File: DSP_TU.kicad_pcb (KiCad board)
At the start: 4 copper layers, 165.1 x 114.3 mm, 83 parts, among them J1 Conn_01x07_Male, J2 Conn_01x08_Male, J3 USB_B, J4 Conn_01x08_Male, J5 1757569, J6 Conn_01x08_Male, J7 Conn_01x08_Male, K1 G3VM-601BY, K2 G3VM-601BY, T1 TY-141P, T2 TY-145P, U1 PIC32MZ0512EFE064-I_PT, U2 TLV2780CDBVT, U3 FT231XS-U, U4 H11AA1, U5 74HCT2G14GW-Q100H, U6 AP2112K-3.3, U7 ATWINC1510-MR210UB, U8 W25X40CLSN

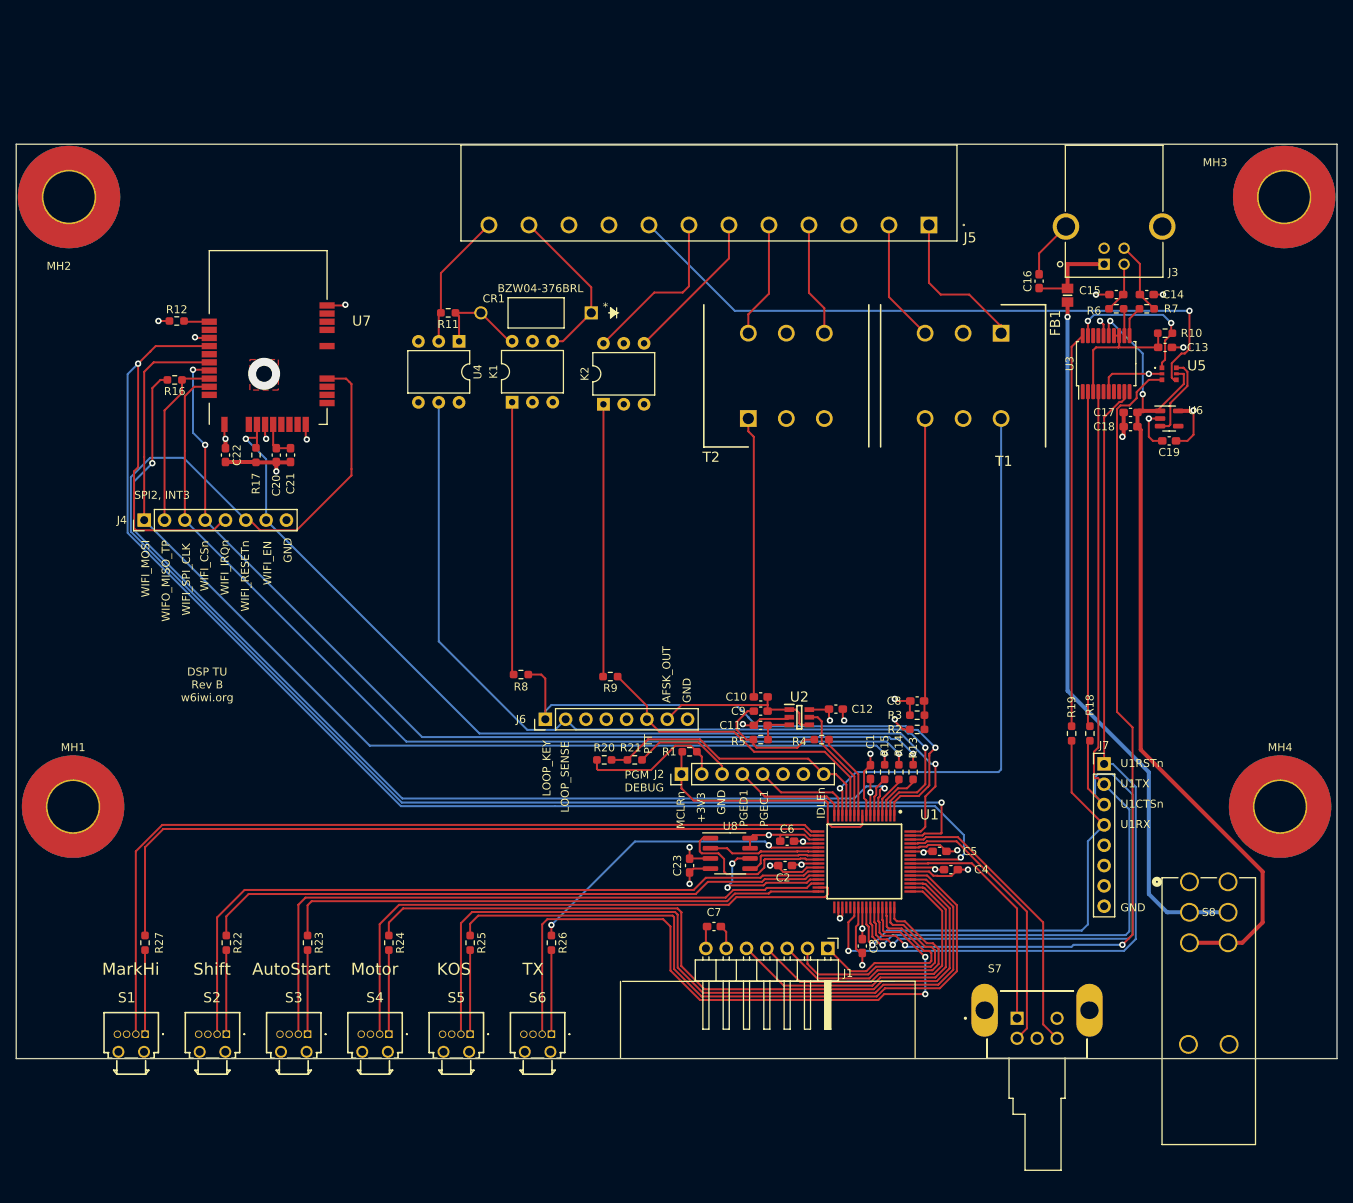
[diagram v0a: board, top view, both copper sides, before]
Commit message: Update all to rev C
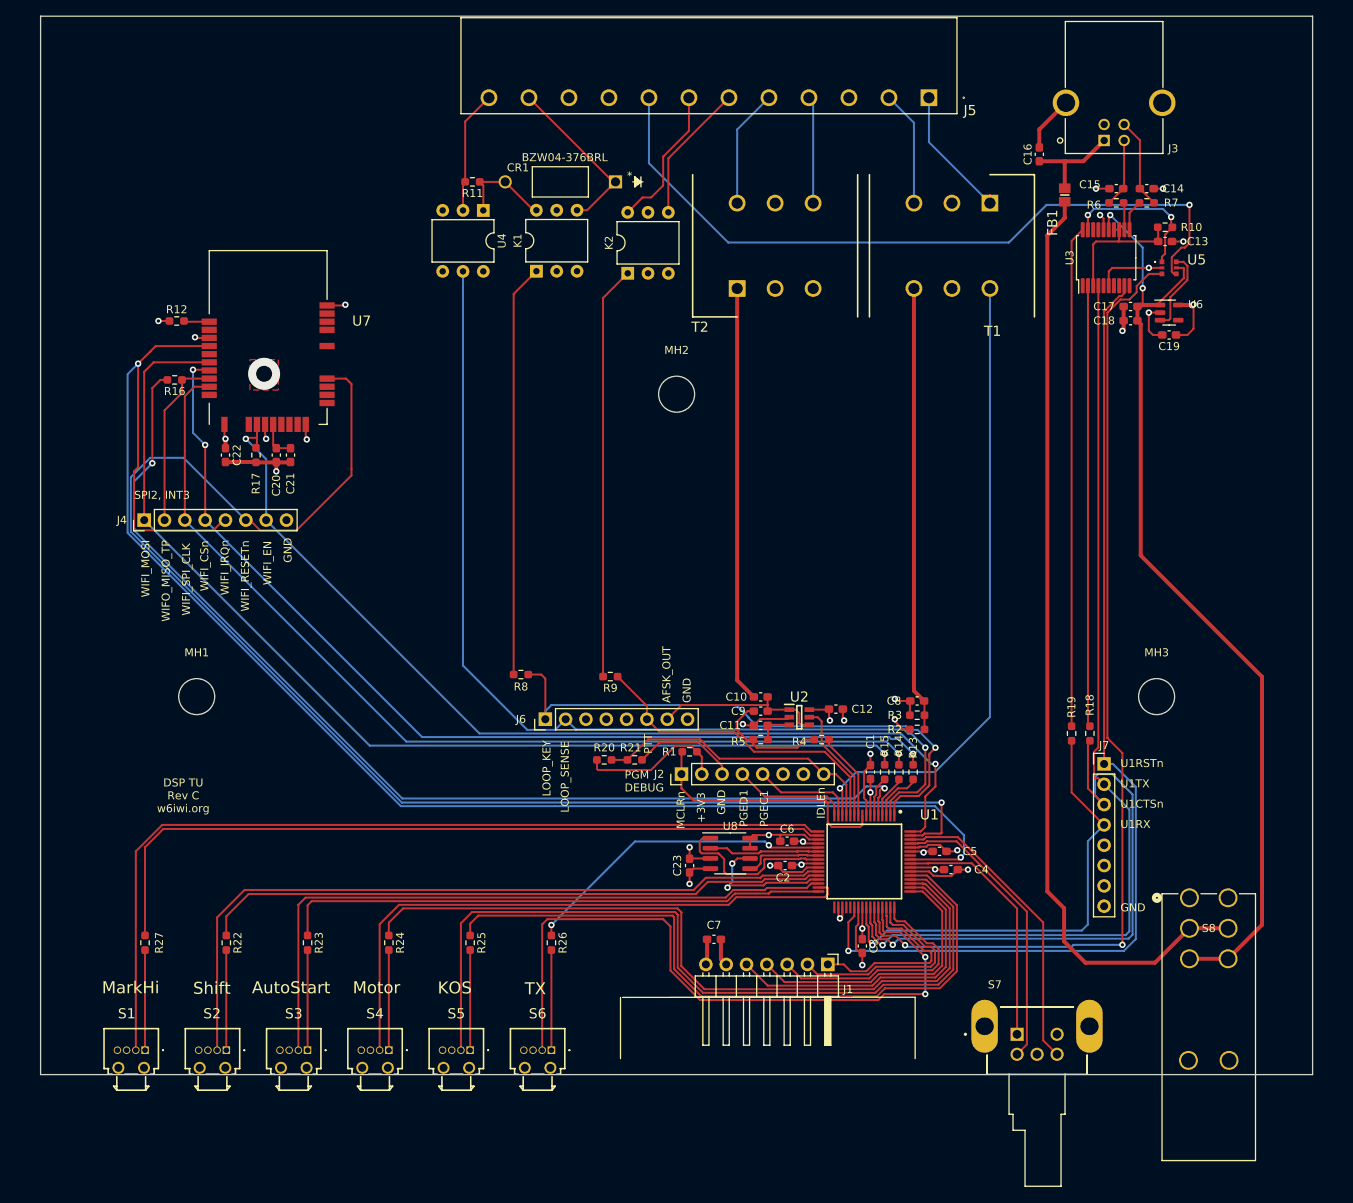
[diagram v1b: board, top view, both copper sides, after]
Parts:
- removed MH4: MountingHole_6.4mm_M6_Pad_TopBottom, MountingHole:MountingHole_6.4mm_M6_Pad_TopBottom
- MH1, MH2, MH3: value MountingHole_6.4mm_M6_Pad_TopBottom -> MountingHole_4.5mm; footprint MountingHole:MountingHole_6.4mm_M6_Pad_TopBottom -> MountingHole:MountingHole_4.5mm
- moved MH2 79.8 mm to (116.6, 60.5)
- moved MH3 64.4 mm to (176.6, 98.3)
- moved MH1 20.7 mm to (56.6, 98.3)
- moved K2 16.7 mm to (110.5, 45.3)
- moved R11 16.7 mm to (91.1, 33.9)
- moved CR1 16.7 mm to (109.0, 33.9)
- moved K1 16.7 mm to (99.1, 45.1)
- moved U4 16.7 mm to (92.4, 37.5)
- moved T1 16.3 mm to (155.8, 36.6)
- moved T2 16.3 mm to (124.2, 47.2)
- moved J5 15.9 mm to (148.1, 23.4)
- moved C16 15.8 mm to (161.9, 30.5)
- moved J3 15.5 mm to (170.0, 28.7)
- moved C18 13.2 mm to (173.3, 51.3)
- moved C13 13.2 mm to (177.6, 41.4)
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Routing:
- net +5V: track 89.1 -> 117.6 mm, vias 1 -> 0
- net Net-(K1-Pad1): track 34.1 -> 51.9 mm
- net Net-(K2-Pad1): track 34.1 -> 51.8 mm
- net Net-(T1-SEC_1): track 39.3 -> 56.2 mm
- net Net-(C10-Pad1): track 35.1 -> 51.9 mm
- net LOOP_SENSE: track 108.9 -> 124.1 mm
- net +5V_SW: track 105.2 -> 119.4 mm
- net U1RTSn: track 114.2 -> 127.4 mm
- net U1TX: track 106.9 -> 120.1 mm
- net Net-(U3-TXD): track 49.4 -> 62.6 mm
- net Net-(U3-RTS#): track 41.9 -> 55.2 mm
- net AUTOSTARTn: track 110.3 -> 123.5 mm
- net Net-(T1-SEC_3): track 68.5 -> 79.5 mm
- net AUTOSTART: track 82.2 -> 92.0 mm
- net PTTb: track 21.3 -> 18.1 mm
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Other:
- board size 165.1 x 114.3 mm -> 159 x 132.3 mm
- board text added: "DSP TU Rev C w6iwi.org"
- board text removed: "DSP TU Rev B w6iwi.org"
